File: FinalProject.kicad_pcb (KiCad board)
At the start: 2 copper layers, 48.3 x 91.4 mm, 22 parts, among them P1 Conn_01x03, P2 Conn_01x02, P3 Conn_01x04, U1 L78L05_TO92, U2 LM339

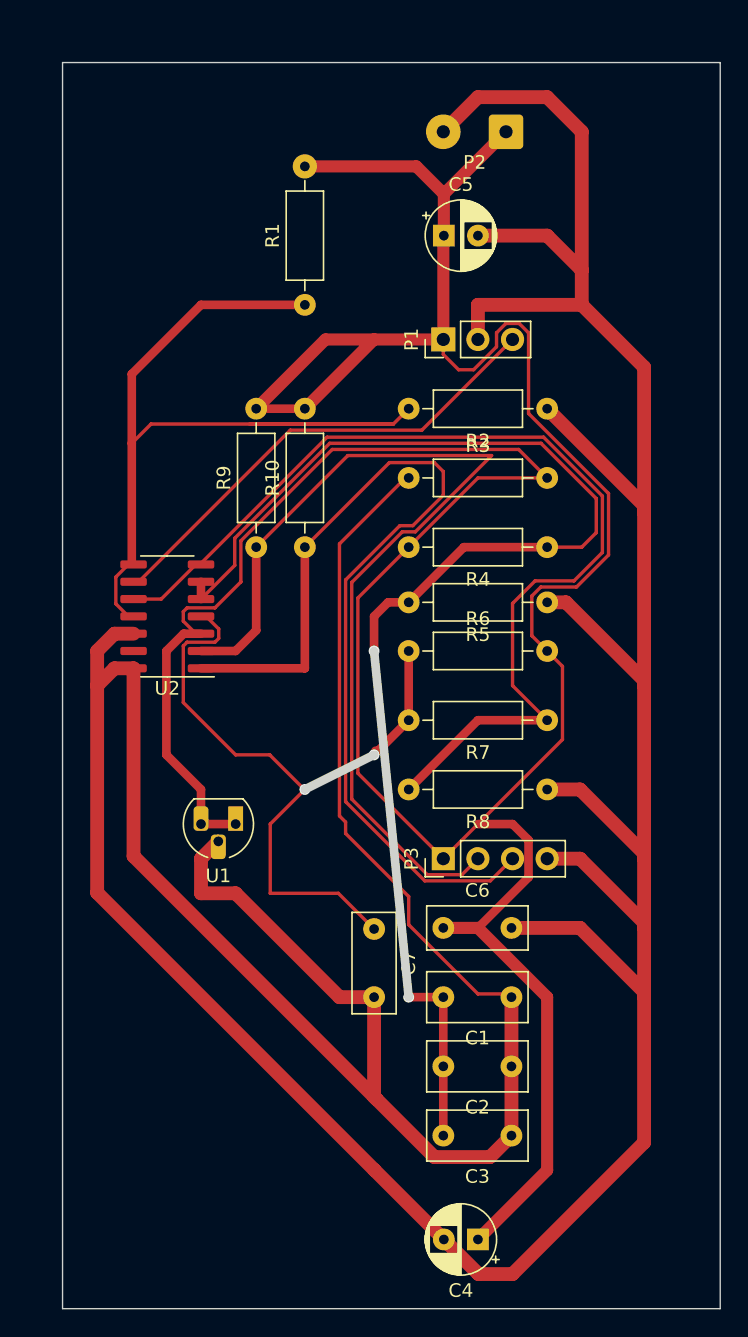
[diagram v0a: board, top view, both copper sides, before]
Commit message: changed file names and deleted previous version
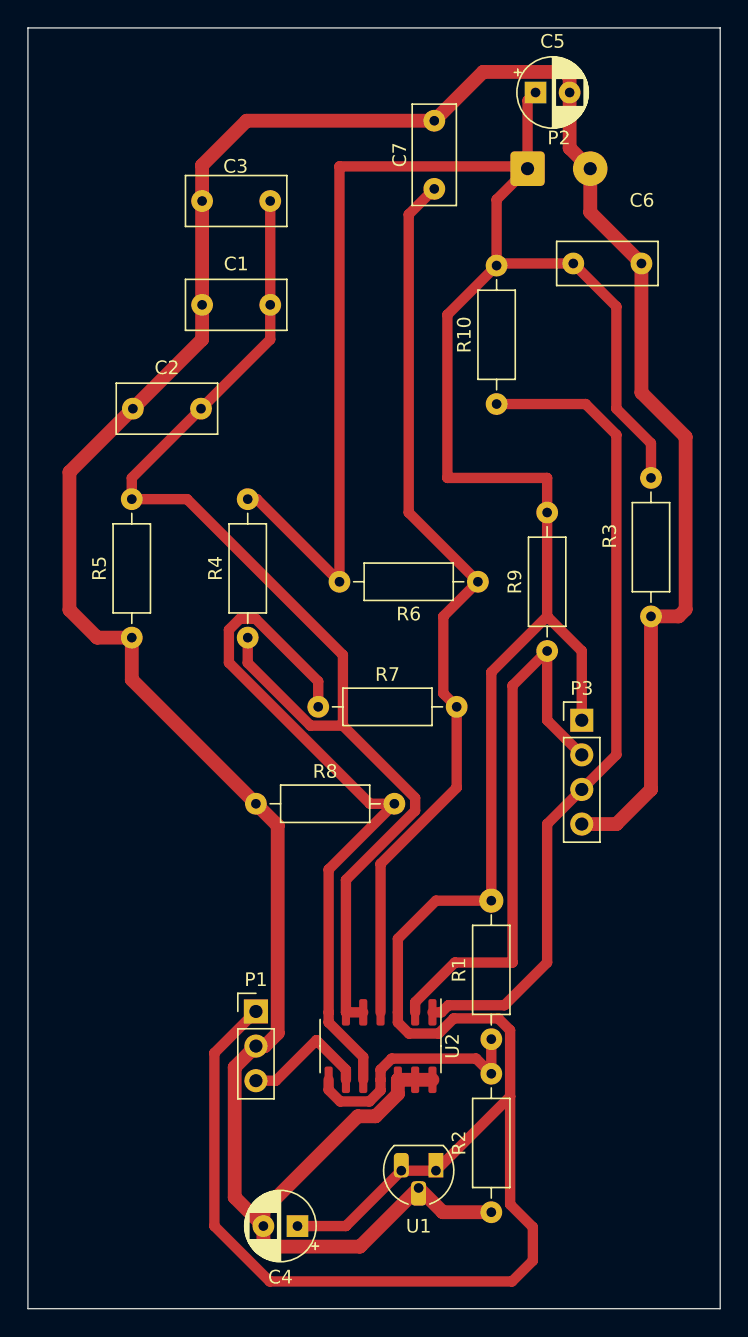
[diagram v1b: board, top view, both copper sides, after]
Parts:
- moved C3 72.2 mm to (144.9, 61.0), turned to 0 degrees
- moved R2 59.1 mm to (166.1, 135.2), turned to 90 degrees
- moved C2 55.7 mm to (139.8, 76.2), turned to 0 degrees
- moved C1 55.6 mm to (144.9, 68.6), turned to 0 degrees
- moved R1 55.6 mm to (166.1, 122.5)
- moved C7 54.5 mm to (161.9, 60.1), turned to 90 degrees
- moved P1 51.2 mm to (148.8, 120.4), turned to 0 degrees
- moved C6 49.7 mm to (172.1, 65.5)
- moved U2 35.2 mm to (158.0, 123.0), turned to -90 degrees
- moved R5 30.6 mm to (139.7, 93.0), turned to 90 degrees
- moved U1 29.4 mm to (162.0, 132.1)
- moved R4 23.0 mm to (148.2, 93.0), turned to 90 degrees
- moved R9 22.7 mm to (170.2, 94.0)
- moved R8 21.4 mm to (148.8, 105.2), turned to 0 degrees
- moved R3 20.5 mm to (177.8, 91.4), turned to 90 degrees
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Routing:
- net GND: track 377.1 -> 225.0 mm
- net Net-(U2C-+): track 66.1 -> 18.2 mm
- net Net-(P3-Pin_2): track 72.9 -> 41.7 mm
- net Net-(P1-Pin_3): track 35.7 -> 9.47 mm
- net Net-(U2B-+): track 75.3 -> 52.8 mm
- net Net-(U2A--): track 46.8 -> 67.1 mm, vias 2 -> 0
- net Net-(U2A-+): track 74.4 -> 88.9 mm, vias 2 -> 0
- net Net-(P3-Pin_3): track 72.6 -> 60.5 mm
- net Net-(P1-Pin_1): track 253.9 -> 260.4 mm
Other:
- board size 48.3 x 91.4 mm -> 50.8 x 94 mm
